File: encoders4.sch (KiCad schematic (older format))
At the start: 45 parts, among them U11 74HCT595, U12 74HC165

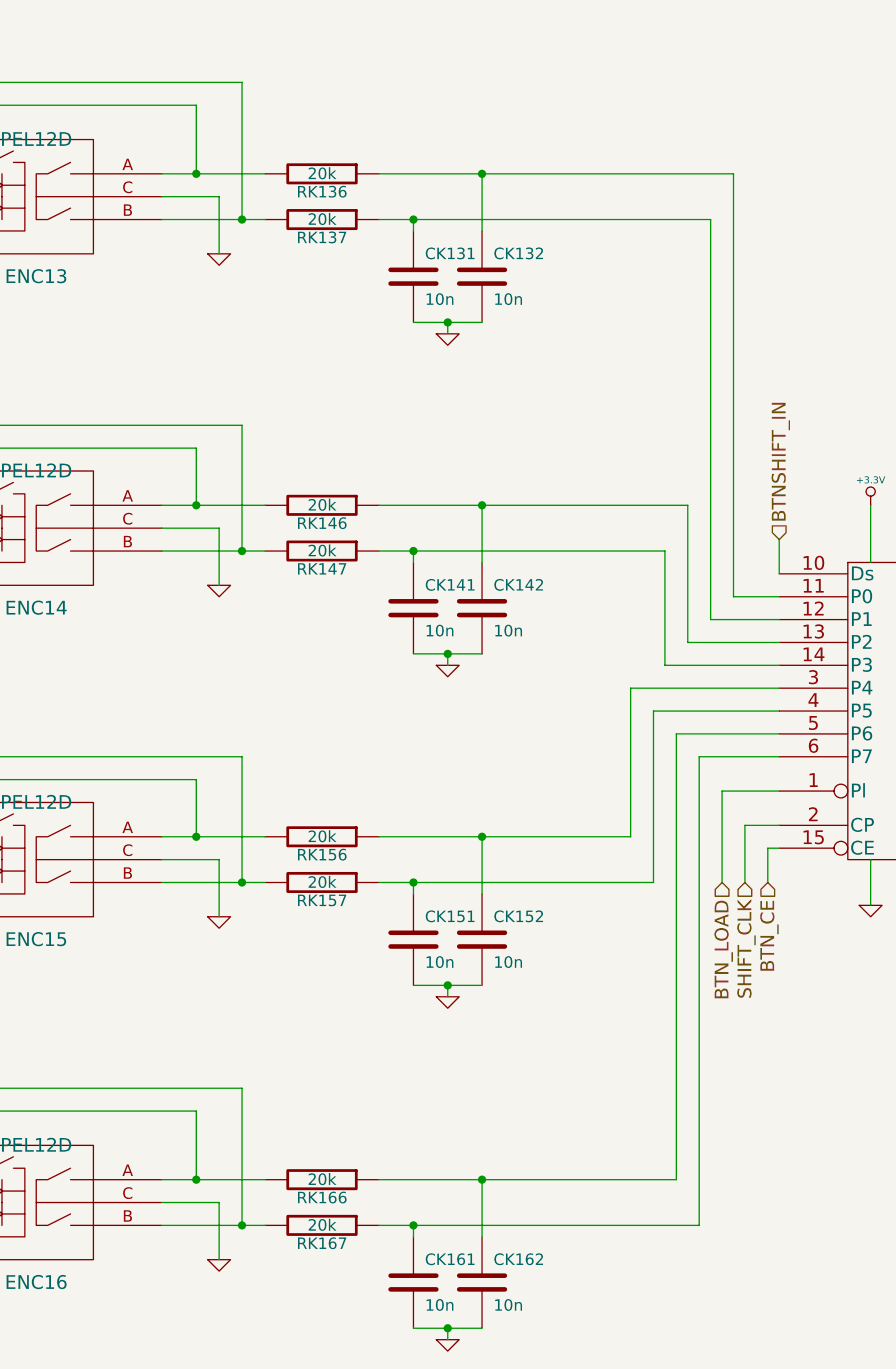
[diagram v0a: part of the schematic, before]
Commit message: Routing.
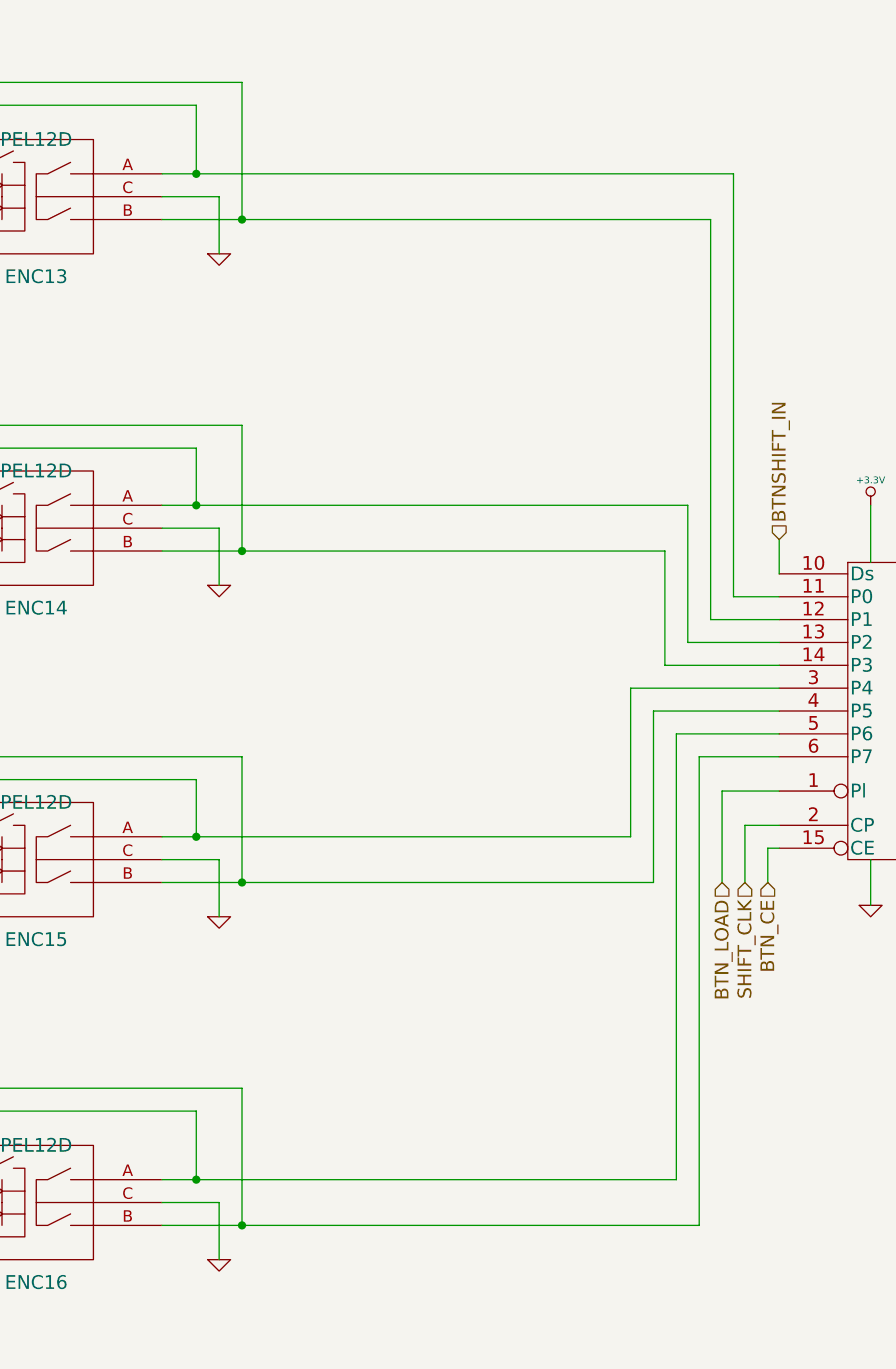
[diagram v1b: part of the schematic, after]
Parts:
- removed CK131, CK132, CK141, CK142, CK151, CK152, CK161, CK162: 10n, symbol C
- removed RK136, RK137, RK146, RK147, RK156, RK157, RK166, RK167: 20k, symbol R
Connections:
- wire segments 173 -> 149
